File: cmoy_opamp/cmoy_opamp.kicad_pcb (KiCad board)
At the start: 2 copper layers, 89.7 x 67.6 mm, 57 parts, among them J1 AudioJack3, J2 AudioJack3, SW1 SPST, U1 MC33178, U2 LMH6642, U3 LMH6642, U4 LMH6642

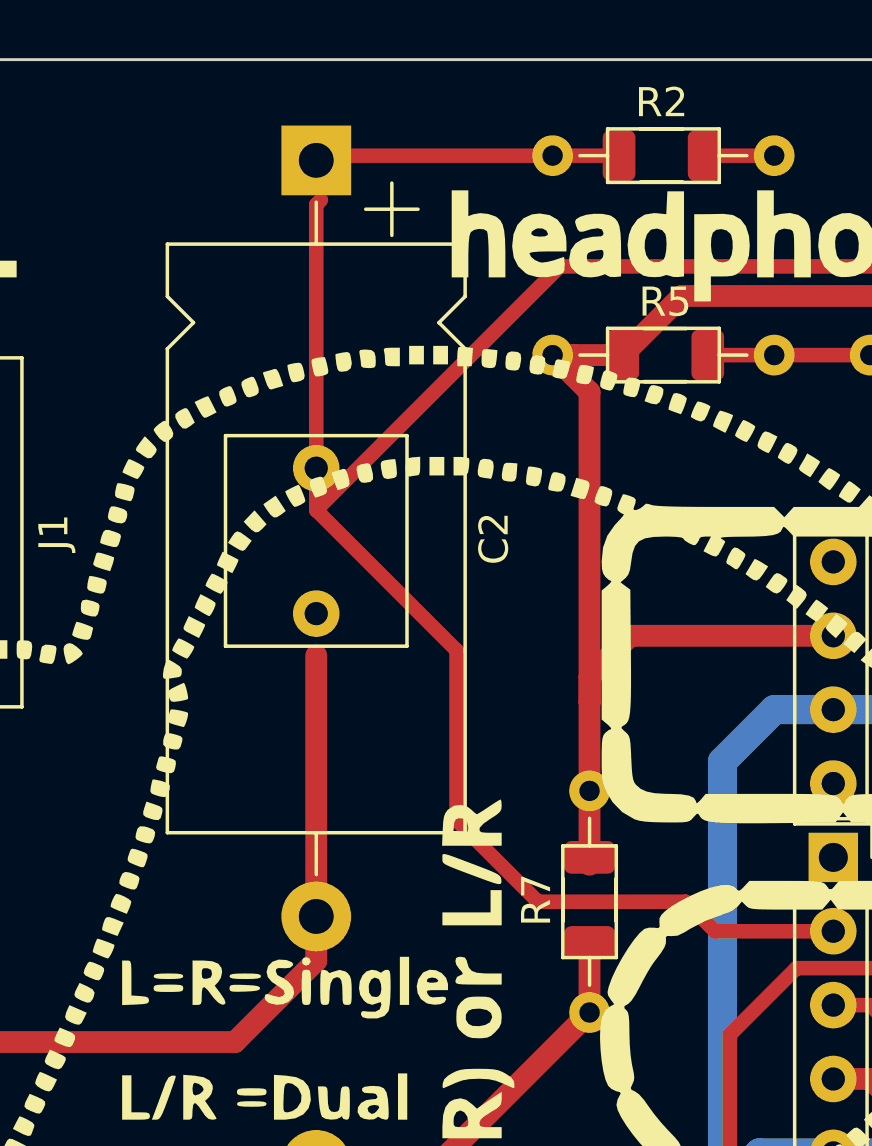
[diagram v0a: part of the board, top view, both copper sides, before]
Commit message: PCB Version ready to order
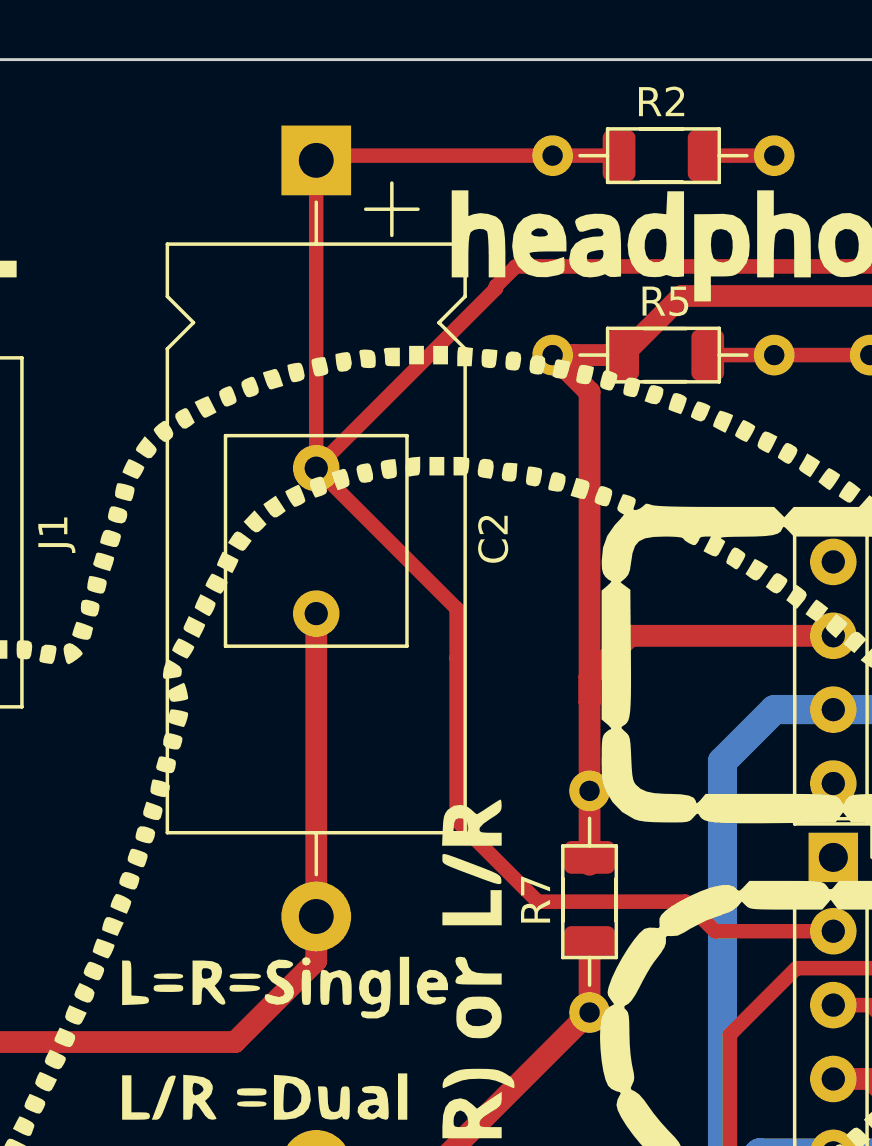
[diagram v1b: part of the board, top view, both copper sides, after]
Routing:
- net Net-(C2-Pad2): track 26.4 -> 27.9 mm
- net /2+: track 125.6 -> 126.3 mm
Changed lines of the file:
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@@
   (segment (start 182.241 46.482) (end 179.832 46.482) (width 0.5) (layer "F.Cu") (net 6))
   (segment (start 180.08 50.292) (end 200.887949 50.292) (width 0.5) (layer "F.Cu") (net 6))
-  (segment (start 171.866 48.006) (end 171.704 48.168) (width 0.5) (layer "F.Cu") (net 6))
+  (segment (start 178.562 50.292) (end 180.08 50.292) (width 0.5) (layer "F.Cu") (net 6))
+  (segment (start 171.704 57.23) (end 177.88 51.054) (width 0.5) (layer "F.Cu") (net 6))
   (segment (start 197.104 88.392) (end 197.866 88.392) (width 0.5) (layer "F.Cu") (net 6))
+  (segment (start 177.88 51.054) (end 177.88 50.974) (width 0.5) (layer "F.Cu") (net 6))
   (segment (start 189.484 73.152) (end 185.42 73.152) (width 0.5) (layer "F.Cu") (net 6))
   (segment (start 179.751 46.482) (end 171.785 46.482) (width 0.5) (layer "F.Cu") (net 6))
   (segment (start 205.994 80.518) (end 197.993 88.519) (width 0.5) (layer "F.Cu") (net 6))
   (segment (start 200.887949 50.292) (end 205.994 55.398051) (width 0.5) (layer "F.Cu") (net 6))
-  (segment (start 176.53 63.494) (end 176.53 69.342) (width 0.5) (layer "F.Cu") (net 6))
   (segment (start 176.53 69.342) (end 179.324 72.136) (width 0.5) (layer "F.Cu") (net 6))
+  (segment (start 176.53 62.056) (end 176.53 63.754) (width 0.5) (layer "F.Cu") (net 6))
   (segment (start 197.866 88.392) (end 197.993 88.519) (width 0.5) (layer "F.Cu") (net 6))
-  (segment (start 171.704 48.168) (end 171.704 58.668) (width 0.5) (layer "F.Cu") (net 6))
   (segment (start 179.324 72.136) (end 184.404 72.136) (width 0.5) (layer "F.Cu") (net 6))
   (segment (start 205.994 55.398051) (end 205.994 80.518) (width 0.5) (layer "F.Cu") (net 6))
-  (segment (start 171.704 58.668) (end 176.53 63.494) (width 0.5) (layer "F.Cu") (net 6))
-  (segment (start 171.704 58.668) (end 180.08 50.292) (width 0.5) (layer "F.Cu") (net 6))
+  (segment (start 171.704 57.23) (end 171.704 46.644) (width 0.5) (layer "F.Cu") (net 6))
+  (segment (start 171.704 57.23) (end 176.53 62.056) (width 0.5) (layer "F.Cu") (net 6))
+  (segment (start 176.53 63.754) (end 176.53 69.342) (width 0.5) (layer "F.Cu") (net 6))
+  (segment (start 177.88 50.974) (end 178.562 50.292) (width 0.5) (layer "F.Cu") (net 6))
   (segment (start 185.42 73.152) (end 184.404 72.136) (width 0.5) (layer "F.Cu") (net 6))
+  (segment (start 156.932 76.962) (end 168.91 76.962) (width 0.75) (layer "F.Cu") (net 7))
   (segment (start 168.91 76.962) (end 171.704 74.168) (width 0.75) (layer "F.Cu") (net 7))
-  (segment (start 156.932 76.962) (end 168.91 76.962) (width 0.75) (layer "F.Cu") (net 7))
-  (segment (start 171.704 63.668) (end 171.704 74.168) (width 0.75) (layer "F.Cu") (net 7))
+  (segment (start 171.704 74.168) (end 171.704 62.23) (width 0.75) (layer "F.Cu") (net 7))
   (segment (start 191.516 92.964) (end 191.516 96.52) (width 1) (layer "F.Cu") (net 8))
   (segment (start 212.852 72.39) (end 212.852 64.516) (width 1) (layer "F.Cu") (net 8))
